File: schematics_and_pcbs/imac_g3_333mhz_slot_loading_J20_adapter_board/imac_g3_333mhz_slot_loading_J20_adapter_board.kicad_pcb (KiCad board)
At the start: 2 copper layers, 82.6 x 45.9 mm, 17 parts, among them J1 DB15_Female_HighDensity, J2 Screw_Terminal_01x06, J20 Conn_02x10_Odd_Even, U1 ATmega328-PU, U2 ATmega328-PU, U3 LCC110, Y1 Crystal, Y2 Crystal

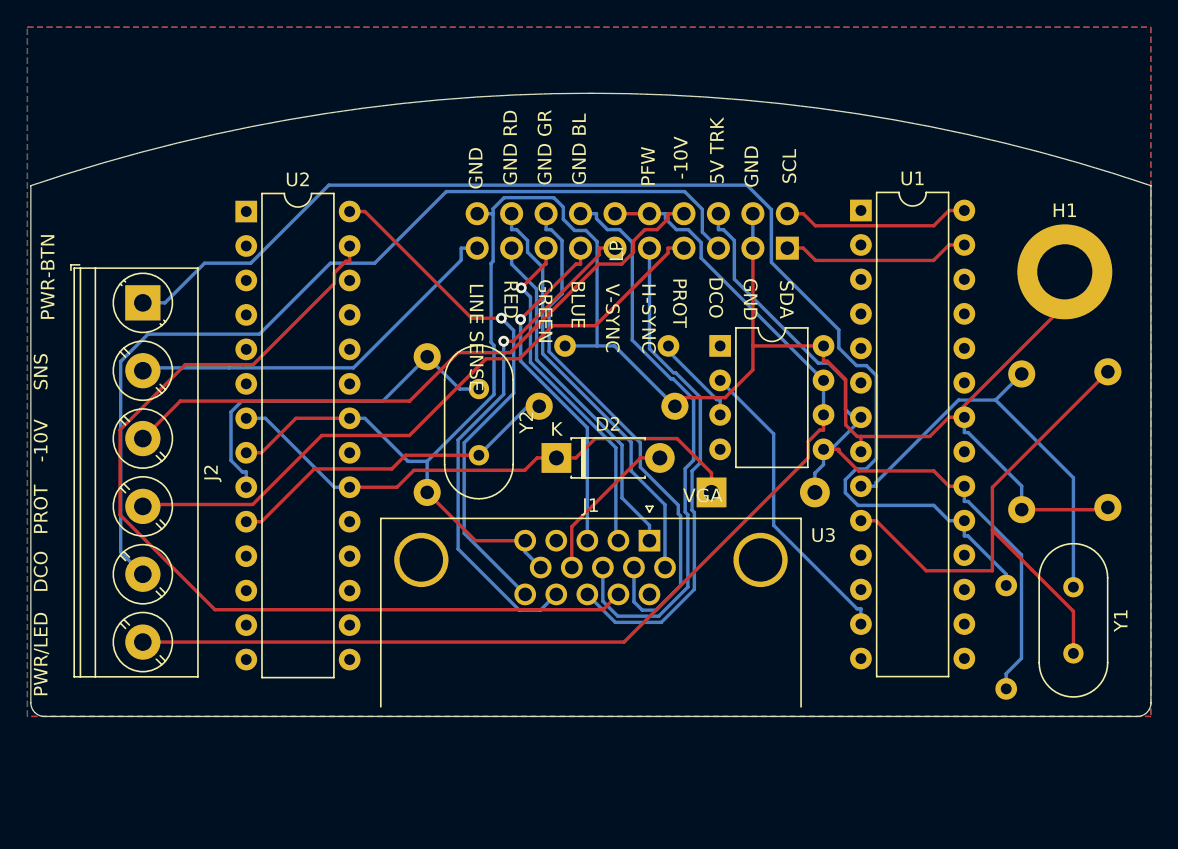
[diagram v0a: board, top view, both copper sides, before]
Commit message: added caps to the board
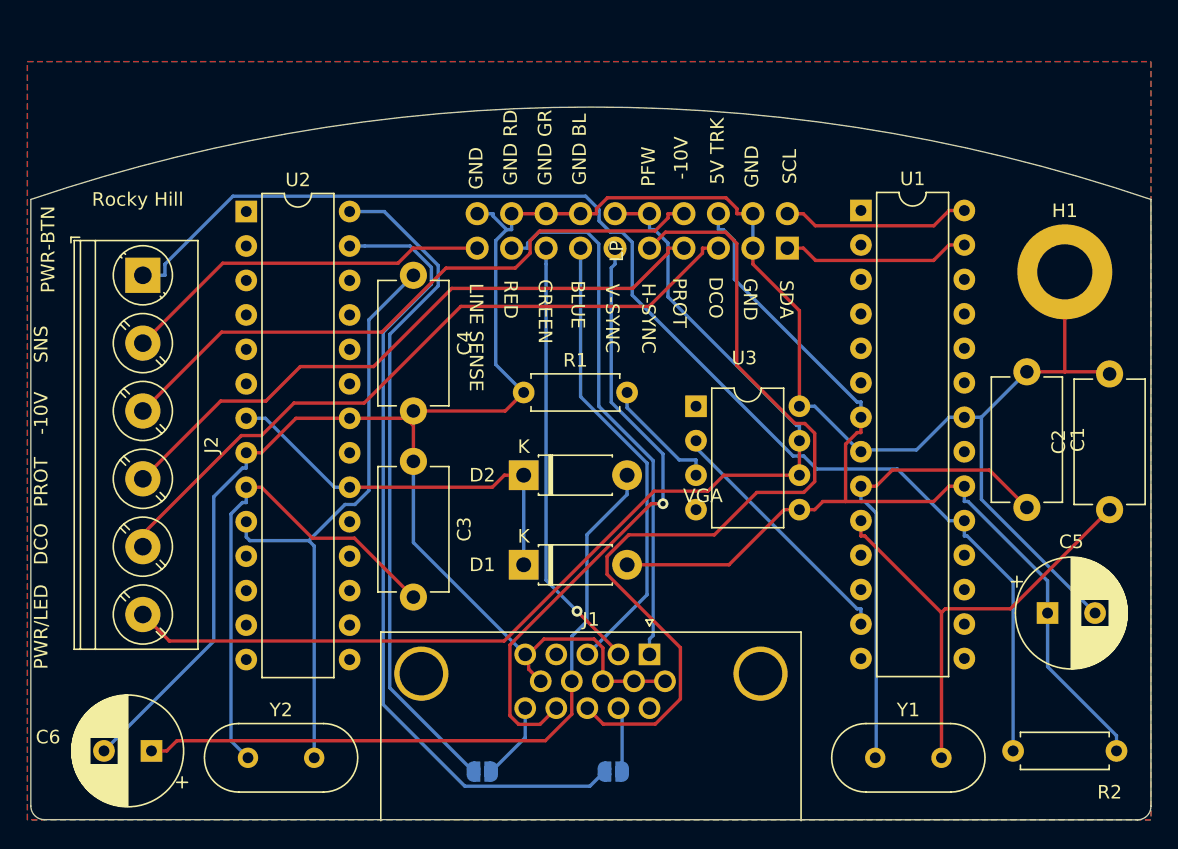
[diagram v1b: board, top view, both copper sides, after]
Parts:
- added C5: 470uF, Capacitor_THT:CP_Radial_D8.0mm_P3.50mm, F.Cu at (208.3, 95.0)
- added C6: 470uF, Capacitor_THT:CP_Radial_D8.0mm_P3.50mm, F.Cu at (142.2, 105.2)
- added JP1: SolderJumper_2_Open, Jumper:SolderJumper-2_P1.3mm_Open_RoundedPad1.0x1.5mm, B.Cu at (176.3, 106.7)
- added JP2: SolderJumper_2_Open, Jumper:SolderJumper-2_P1.3mm_Open_RoundedPad1.0x1.5mm, B.Cu at (166.6, 106.7)
- C1, C2, C3, C4, D1, R1, R2: moved to F.Cu
- moved Y2 32.1 mm to (149.4, 105.7), turned to 0 degrees
- moved Y1 19.3 mm to (195.6, 105.7), turned to 0 degrees
- moved D1 14.8 mm to (169.7, 91.4)
- moved C4 13.4 mm to (161.5, 70.1), turned to 270 degrees
- moved R2 12.2 mm to (205.7, 105.2), turned to 0 degrees
- moved C1 10.2 mm to (206.8, 77.2), turned to 270 degrees
- moved C2 10.2 mm to (212.9, 87.4), turned to 90 degrees
- moved J1 8.38 mm to (178.9, 98.0)
- moved U3 4.79 mm to (182.4, 79.8)
- moved R1 4.59 mm to (169.7, 78.7)
- moved D2 2.73 mm to (169.7, 84.8)
- moved C3 2.50 mm to (161.5, 83.8), turned to 270 degrees
- moved J2 2.03 mm to (141.6, 70.1)
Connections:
- J1 pad 12: /COMPUTER_SDA -> Net-(J1-Pad12)
- J1 pad 15: /COMPUTER_SCL -> Net-(J1-Pad15)
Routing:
- net GND: track 262.0 -> 190.0 mm
- net /COMPUTER_5V: track 11.6 -> 51.4 mm
- net /H_SYNC: track 36.9 -> 66.1 mm
- net /5V_TRICKLE: track 57.2 -> 78.1 mm
- net Net-(C4-Pad1): track 25.1 -> 45.2 mm
- net /DCO: track 68.3 -> 52.3 mm
- net /RED: track 25.8 -> 39.5 mm
- net /COMPUTER_SCL: track 38.5 -> 49.5 mm, vias 1 -> 0
- net Net-(D1-Pad1): track 40.4 -> 29.5 mm
- net /COMPUTER_SDA: track 70.0 -> 59.6 mm
- net Net-(C3-Pad2): track 27.1 -> 36.8 mm
- net /BLUE: track 25.6 -> 33.8 mm, vias 1 -> 0
- net /V_SYNC: track 37.6 -> 45.5 mm
- net /GREEN: track 25.3 -> 32.1 mm
- net Net-(J1-Pad15): track 0.00 -> 5.72 mm
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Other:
- board size 82.6 x 45.9 mm -> 82.6 x 52.5 mm
- board text added: "Rocky Hill"
- board text added: "iMac G3 DV VGA on/off adapter"
- board text added: "solder jumpers to send EDID"
